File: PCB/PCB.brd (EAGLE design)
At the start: 41 x 41 mm, 55 parts, among them Q1 BSS138, Q2 BSS138, Q3 BSS138, Q4 BSS138

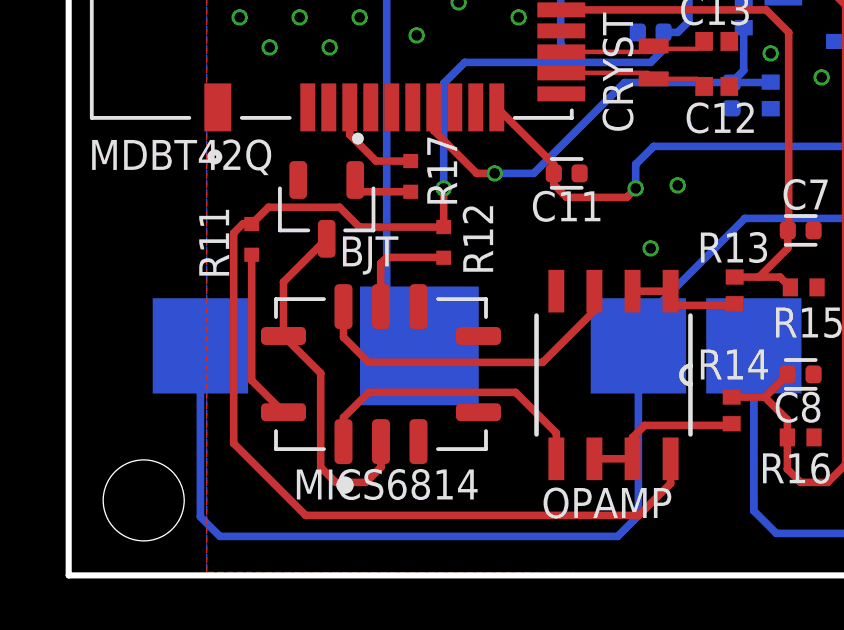
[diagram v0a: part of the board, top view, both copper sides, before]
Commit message: Modifiche codice analisi
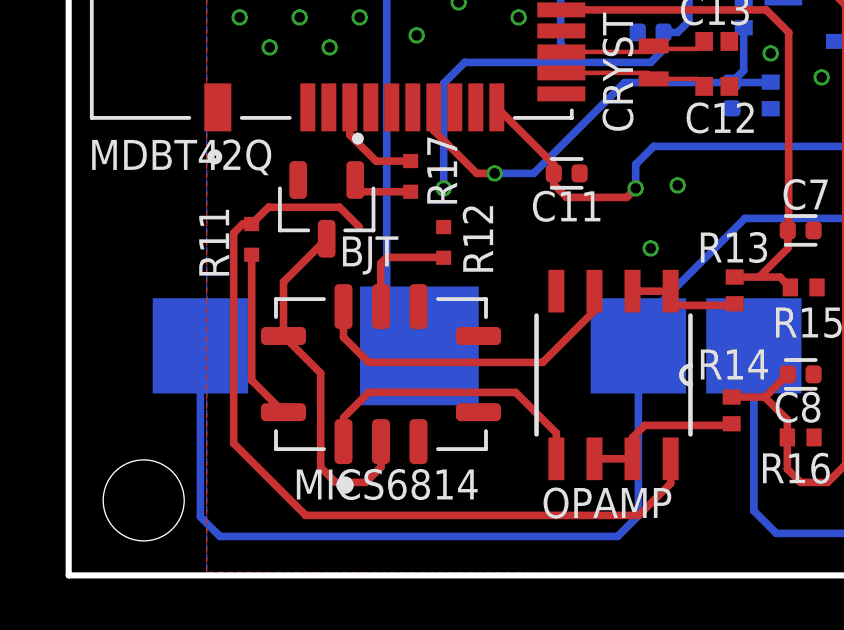
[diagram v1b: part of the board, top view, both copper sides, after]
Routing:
- net 5V: track 81.1 -> 77.0 mm
- net N$3: track 9.66 -> 8.86 mm
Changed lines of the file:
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@@
 <contactref element="R9" pad="2"/>
 <contactref element="R11" pad="2"/>
-<contactref element="R12" pad="2"/>
-<wire x1="22.5" y1="38.612" x2="22.5" y2="39.9" width="0.254" layer="1"/>
-<wire x1="22.5" y1="38.612" x2="19.688" y2="38.612" width="0.254" layer="1"/>
 <wire x1="19.0294" y1="39.2706" x2="19.688" y2="38.612" width="0.254" layer="1"/>
 <wire x1="15.5" y1="31.4" x2="15.5" y2="38.412" width="0.254" layer="1"/>
@@
 <wire x1="30.5" y1="56.9" x2="30.5" y2="57.2" width="0.254" layer="1"/>
 <wire x1="30.5" y1="57.2" x2="30.857" y2="57.557" width="0.254" layer="1"/>
+<contactref element="R12" pad="2"/>
+<wire x1="22.5" y1="38.612" x2="22.5" y2="39.9" width="0" layer="19" extent="1-1"/>
+<wire x1="19.688" y1="38.612" x2="22.5" y2="38.612" width="0" layer="19" extent="1-1"/>
 </signal>
 <signal name="SDA5">
@@
 <wire x1="44.15" y1="48" x2="38.7285" y2="42.5785" width="0.1524" layer="1"/>
 <wire x1="38.7285" y1="42.5785" x2="37.5785" y2="42.5785" width="0.1524" layer="1"/>
-</signal>
-<signal name="N$6">
-<contactref element="MICS6814" pad="A"/>
-<contactref element="OPAMP" pad="5"/>
-<wire x1="26.255" y1="30.886" x2="26.255" y2="31.745" width="0.254" layer="1"/>
-<wire x1="24.9" y1="33.1" x2="26.255" y2="31.745" width="0.254" layer="1"/>
-<wire x1="19.16" y1="31.46" x2="19.16" y2="32.26" width="0.254" layer="1"/>
-<wire x1="20" y1="33.1" x2="24.9" y2="33.1" width="0.254" layer="1"/>
-<wire x1="19.16" y1="32.26" x2="20" y2="33.1" width="0.254" layer="1"/>
 </signal>
 <signal name="N$10">
@@
 <wire x1="20.41" y1="31.46" x2="20.41" y2="30.61" width="0.254" layer="1"/>
 </signal>
+<signal name="N$3">
+<contactref element="MICS6814" pad="A"/>
+<contactref element="OPAMP" pad="5"/>
+<wire x1="26.255" y1="30.886" x2="26.255" y2="31.745" width="0.254" layer="1"/>
+<wire x1="24.9" y1="33.1" x2="26.255" y2="31.745" width="0.254" layer="1"/>
+<wire x1="20" y1="33.1" x2="24.9" y2="33.1" width="0.254" layer="1"/>
+<wire x1="19.16" y1="32.26" x2="20" y2="33.1" width="0.254" layer="1"/>
+<wire x1="19.16" y1="32.26" x2="19.16" y2="31.46" width="0" layer="19" extent="1-1"/>
+</signal>
 </signals>
